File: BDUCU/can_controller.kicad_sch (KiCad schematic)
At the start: 11 parts, among them U10 TJA1050T_CM_118, U11 MCP2515-xST, Y2 20MHz

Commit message: bducu scheme done, waiting for check
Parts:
- U10: footprint Package_SO:SOIC-8_3.9x4.9mm_P1.27mm -> RMC_SO:SOIC-8_3.9x4.9mm_P1.27mm_RMC_Handsolder
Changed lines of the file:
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@@
 			)
 		)
-		(property "Footprint" "Package_SO:SOIC-8_3.9x4.9mm_P1.27mm"
+		(property "Footprint" "RMC_SO:SOIC-8_3.9x4.9mm_P1.27mm_RMC_Handsolder"
 			(at 181.356 89.662 0)
 			(effects
@@
 			)
 		)
-		(property "Description" "\n1/1 Transceiver Half CANbus 8-SO\n"
+		(property "Description" "1/1 Transceiver Half CANbus 8-SO"
 			(at 181.356 89.662 0)
 			(effects

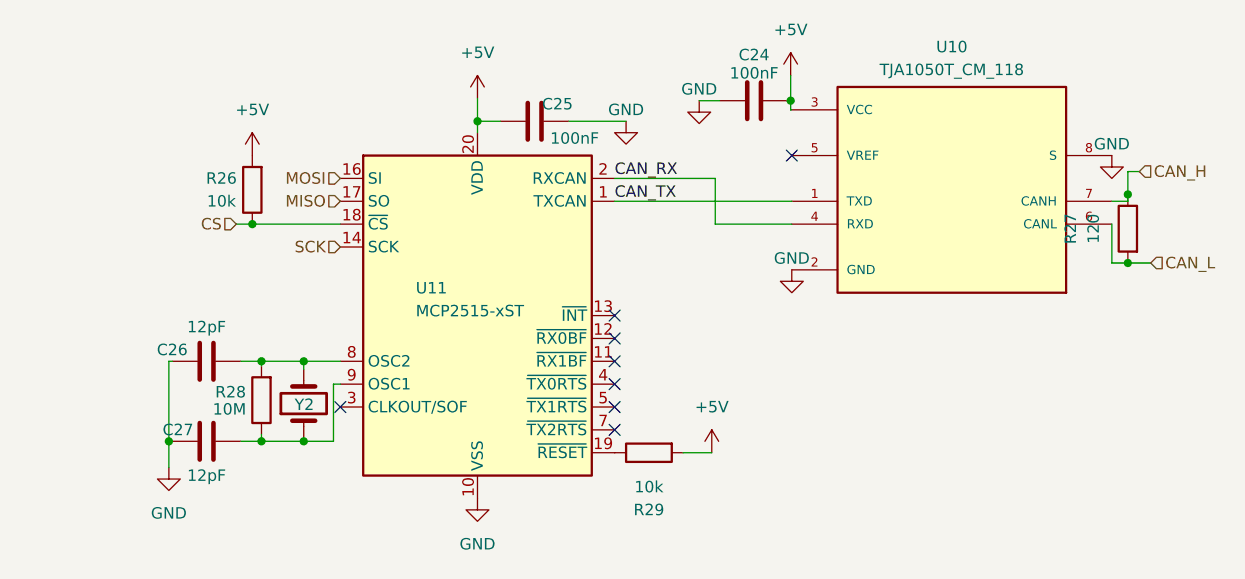
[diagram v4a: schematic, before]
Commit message: I am Nicholas Chan (lesbian version)
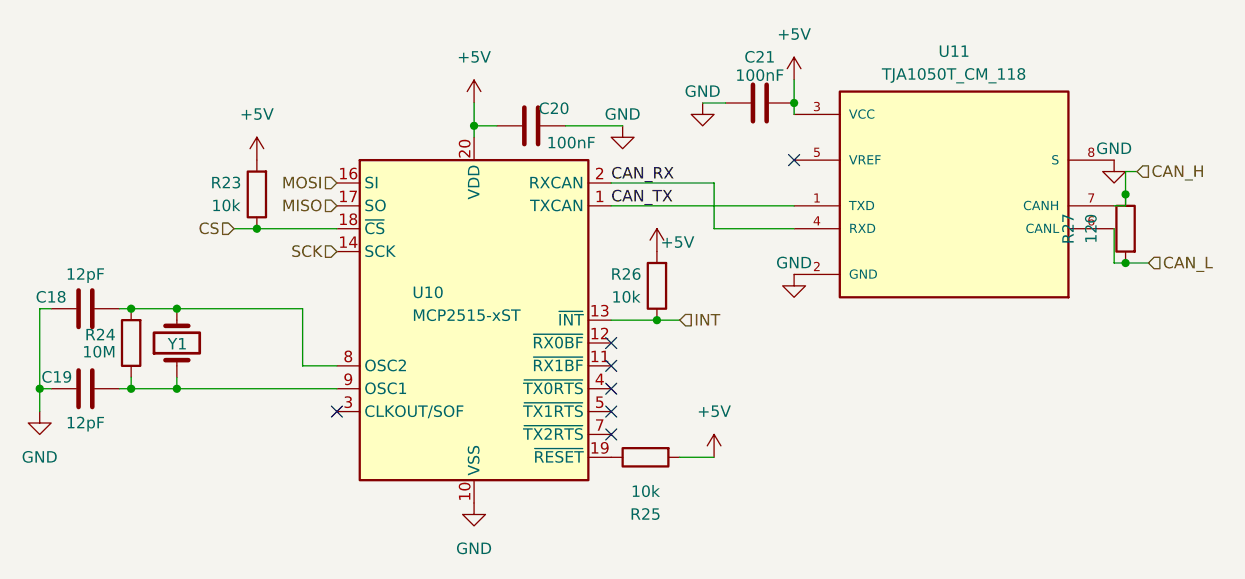
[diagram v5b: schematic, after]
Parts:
- added R23: 10k, RMC_Resistor:R_0805_2012Metric_Pad1.20x1.40mm_HandSolder_L, symbol Device:R
- renumbered C26 to C18, C27 to C19, C25 to C20, C24 to C21, R28 to R24, R29 to R25, U11 to U10, U10 to U11, Y2 to Y1
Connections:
- net +5V: now also R23.2
- net CS: now also R23.1; no longer R26.1
- net INT: now reaches U10.13 (~{INT})
- net INT: now also R26.1
- no-connect marks 8 -> 7
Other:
- moved on the sheet: C18, C19, C20, C21, R24, R25, R26, U10, U11, Y1
